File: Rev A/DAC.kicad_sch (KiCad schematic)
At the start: 19 parts, among them U6 74HC595

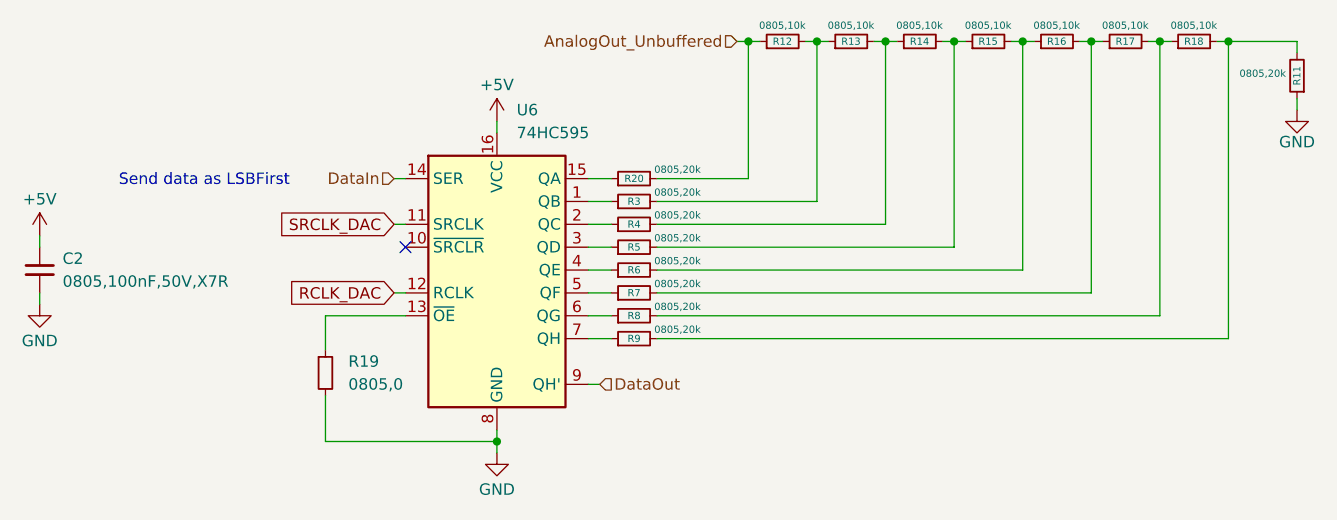
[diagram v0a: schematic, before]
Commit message: added more schematic stuffs
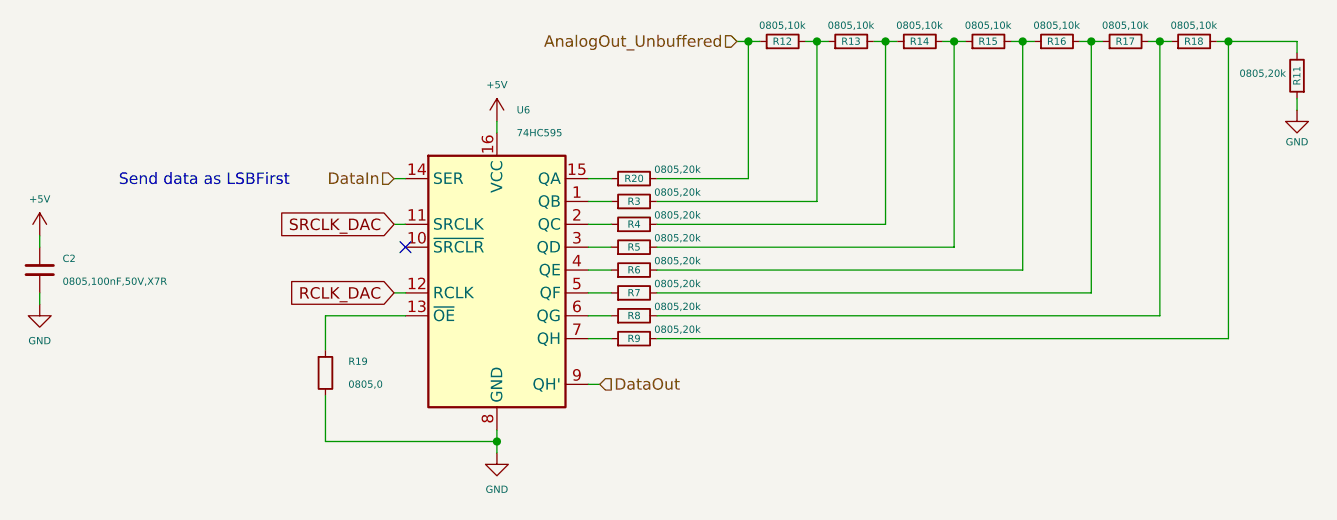
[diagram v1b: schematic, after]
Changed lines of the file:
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@@
 			(effects
 				(font
-					(size 1.27 1.27)
+					(size 0.8 0.8)
 				)
 				(hide yes)
@@
 			(effects
 				(font
-					(size 1.27 1.27)
+					(size 0.8 0.8)
 				)
 			)
@@
 			(effects
 				(font
-					(size 1.27 1.27)
+					(size 0.8 0.8)
 				)
 				(hide yes)
@@
 			(effects
 				(font
-					(size 1.27 1.27)
+					(size 0.8 0.8)
 				)
 			)
@@
 			(effects
 				(font
-					(size 1.27 1.27)
+					(size 0.8 0.8)
 				)
 				(justify left)
@@
 			(effects
 				(font
-					(size 1.27 1.27)
+					(size 0.8 0.8)
 				)
 				(justify left)
@@
 			(effects
 				(font
-					(size 1.27 1.27)
+					(size 0.8 0.8)
 				)
 				(hide yes)
@@
 			(effects
 				(font
-					(size 1.27 1.27)
+					(size 0.8 0.8)
 				)
 			)
@@
 			(effects
 				(font
-					(size 1.27 1.27)
+					(size 0.8 0.8)
 				)
 				(justify left)
@@
 			(effects
 				(font
-					(size 1.27 1.27)
+					(size 0.8 0.8)
 				)
 				(justify left)
@@
 			(effects
 				(font
-					(size 1.27 1.27)
+					(size 0.8 0.8)
 				)
 				(hide yes)
@@
 			(effects
 				(font
-					(size 1.27 1.27)
+					(size 0.8 0.8)
 				)
 			)
@@
 			(effects
 				(font
-					(size 1.27 1.27)
+					(size 0.8 0.8)
 				)
 				(hide yes)
@@
 			(effects
 				(font
-					(size 1.27 1.27)
+					(size 0.8 0.8)
 				)
 			)
@@
 			(effects
 				(font
-					(size 1.27 1.27)
+					(size 0.8 0.8)
 				)
 				(justify left)
@@
 			(effects
 				(font
-					(size 1.27 1.27)
+					(size 0.8 0.8)
 				)
 				(justify left)
